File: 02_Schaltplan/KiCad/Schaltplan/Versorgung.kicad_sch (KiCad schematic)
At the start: 31 parts, among them J5 9V_Batt, Q2 Si2301, SW3 PWR ON/OFF, U7 TPS_54331

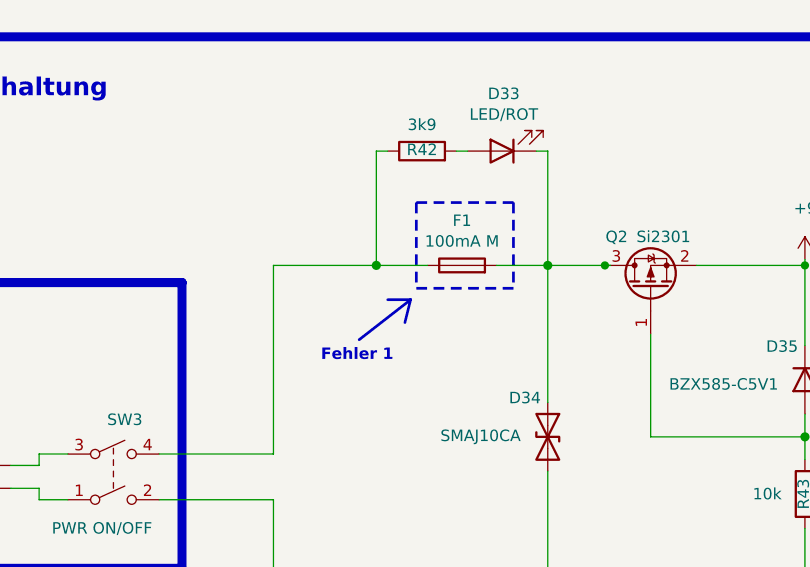
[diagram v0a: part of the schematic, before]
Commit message: ADD
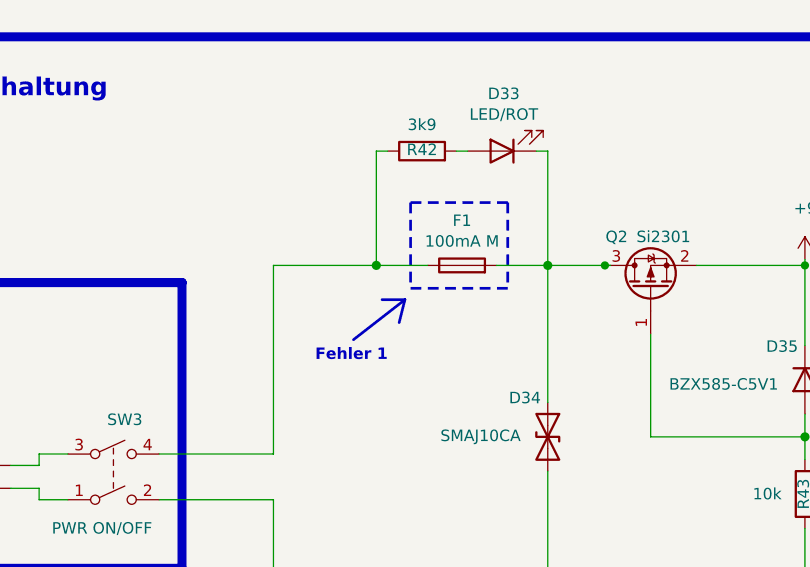
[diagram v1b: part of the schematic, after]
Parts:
- D33, D36, D38: Stromaufnahme (none) -> 1mA
- U7: Stromaufnahme (none) -> 110uA
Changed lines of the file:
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@@
     (stroke (width 1) (type solid) (color 0 255 0 1))
   )
-  (polyline (pts (xy 81.28 116.205) (xy 86.995 111.76))
+  (polyline (pts (xy 80.645 116.205) (xy 86.36 111.76))
     (stroke (width 0.3) (type solid) (color 0 0 255 1))
   )
-  (polyline (pts (xy 86.36 114.3) (xy 86.995 111.76))
+  (polyline (pts (xy 85.725 114.3) (xy 86.36 111.76))
     (stroke (width 0.3) (type solid) (color 0 0 255 1))
   )
-  (polyline (pts (xy 86.995 111.76) (xy 84.455 111.76))
+  (polyline (pts (xy 86.36 111.76) (xy 83.82 111.76))
     (stroke (width 0.3) (type solid) (color 0 0 255 1))
   )
-  (polyline (pts (xy 87.63 100.965) (xy 87.63 110.49))
+  (polyline (pts (xy 86.995 100.965) (xy 86.995 110.49))
     (stroke (width 0.3) (type dash_dot) (color 0 0 255 1))
   )
-  (polyline (pts (xy 87.63 100.965) (xy 98.425 100.965))
+  (polyline (pts (xy 86.995 100.965) (xy 97.79 100.965))
     (stroke (width 0.3) (type dash_dot) (color 0 0 255 1))
   )
-  (polyline (pts (xy 98.425 100.965) (xy 98.425 110.49))
+  (polyline (pts (xy 97.79 100.965) (xy 97.79 110.49))
     (stroke (width 0.3) (type dash_dot) (color 0 0 255 1))
   )
-  (polyline (pts (xy 98.425 110.49) (xy 87.63 110.49))
+  (polyline (pts (xy 97.79 110.49) (xy 86.995 110.49))
     (stroke (width 0.3) (type dash_dot) (color 0 0 255 1))
   )
@@
     (effects (font (size 2 2) (thickness 0.4) bold) (justify right bottom))
   )
-  (text "Fehler 1" (at 85.09 118.745 180)
+  (text "Fehler 1" (at 84.455 118.745 180)
     (effects (font (size 1.27 1.27) (thickness 0.254) bold) (justify right bottom))
   )
@@
       (effects (font (size 1.27 1.27)) hide)
     )
+    (property "Stromaufnahme" "1mA" (id 4) (at 97.155 95.25 0)
+      (effects (font (size 1.27 1.27)) hide)
+    )
     (pin "1")
     (pin "2")
@@
       (effects (font (size 1.27 1.27)) hide)
     )
+    (property "Stromaufnahme" "1mA" (id 4) (at 155.575 133.35 0)
+      (effects (font (size 1.27 1.27)) hide)
+    )
     (pin "1")
     (pin "2")
@@
     )
     (property "Mouser" "604-APT1608LZGCK" (id 4) (at 317.5 142.875 0)
+      (effects (font (size 1.27 1.27)) hide)
+    )
+    (property "Stromaufnahme" "1mA" (id 4) (at 317.5 142.875 0)
       (effects (font (size 1.27 1.27)) hide)
     )
@@
       (effects (font (size 1.27 1.27)) hide)
     )
+    (property "Stromaufnahme" "110uA" (id 4) (at 240.03 123.19 0)
+      (effects (font (size 1.27 1.27)) hide)
+    )
